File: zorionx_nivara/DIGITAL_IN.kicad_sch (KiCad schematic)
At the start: 8 parts, among them U5 LTV-357T, U6 LTV-357T

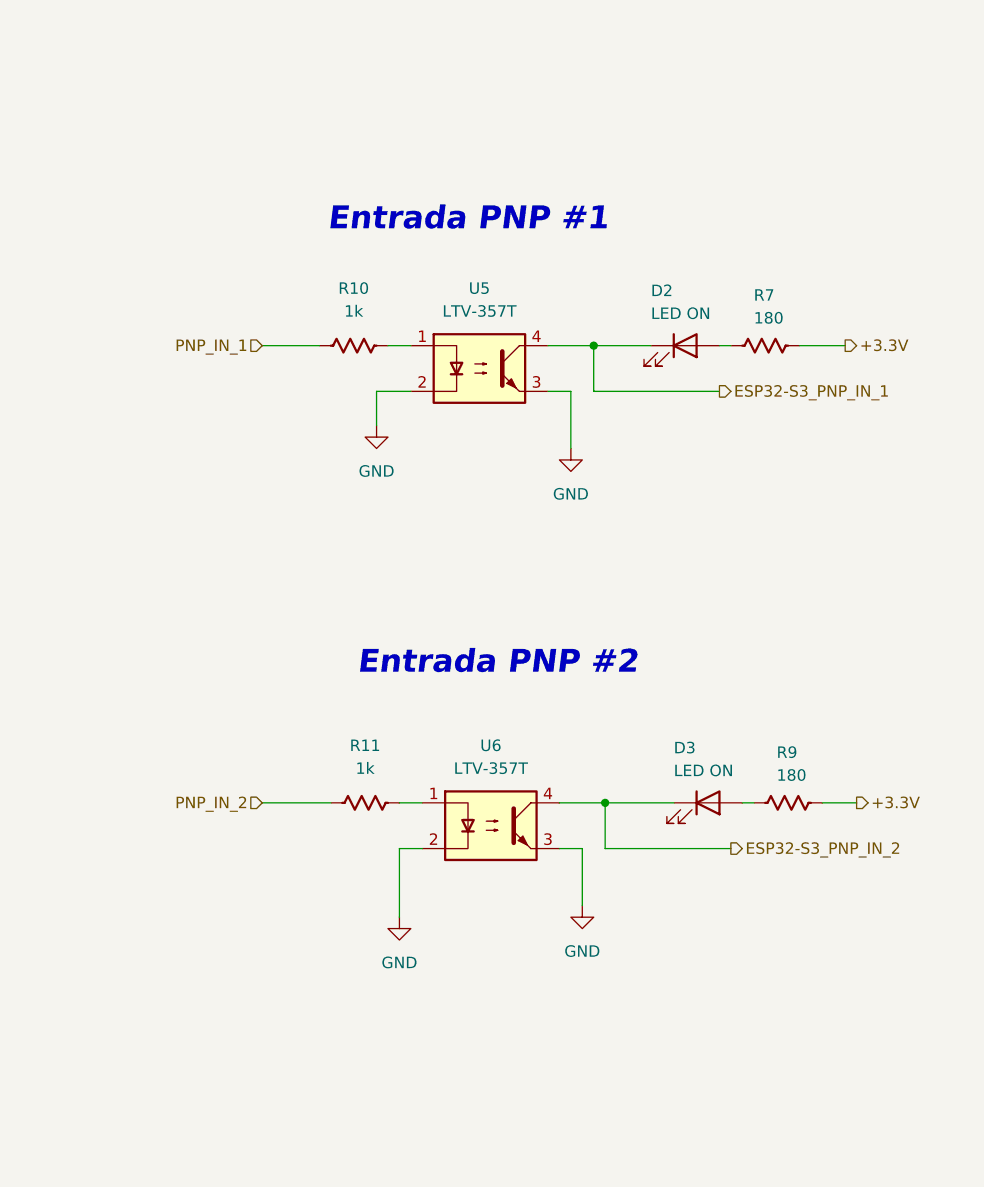
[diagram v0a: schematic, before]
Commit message: ultimo commit 1
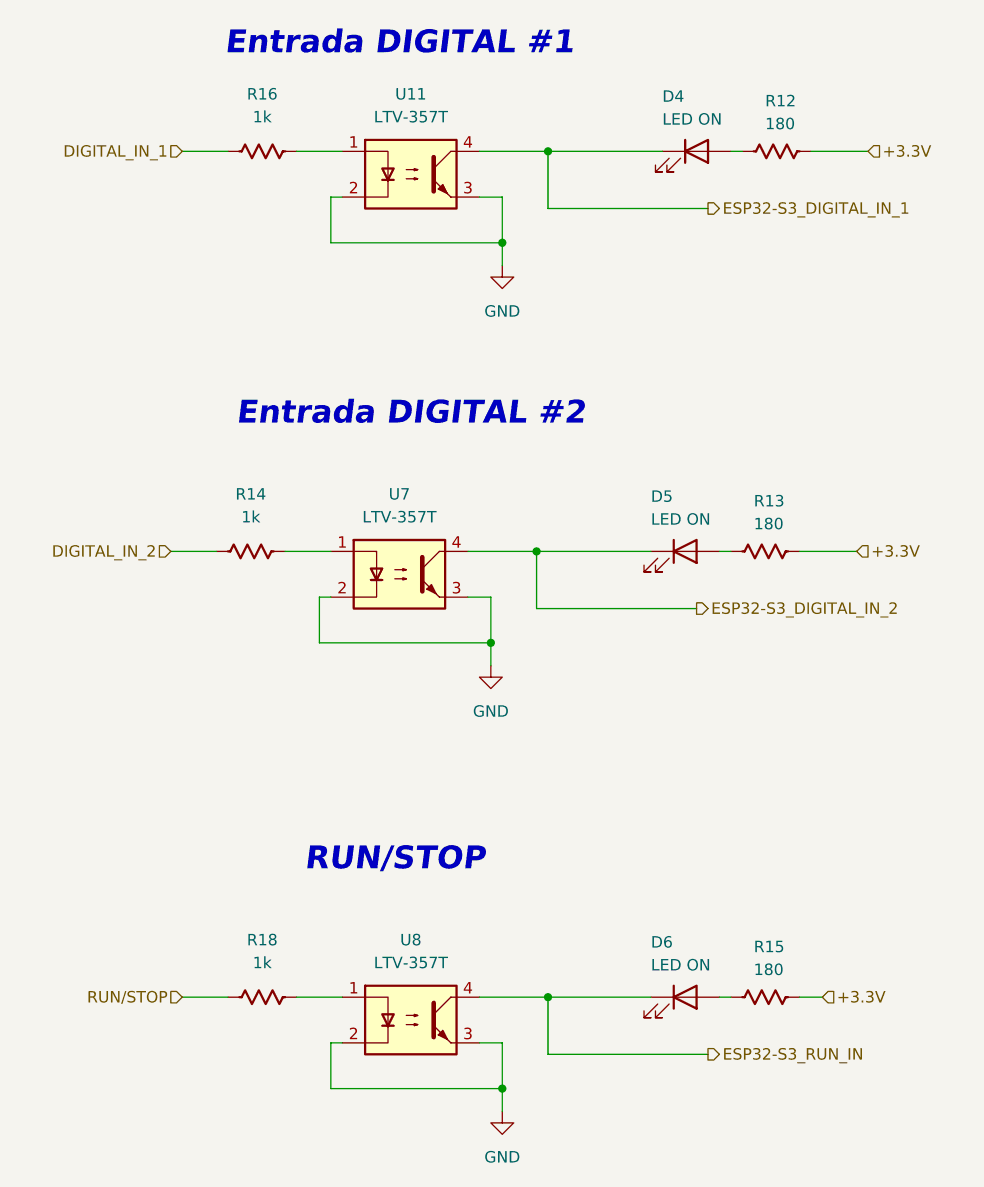
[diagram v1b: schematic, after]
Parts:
- removed D2, D3: LED ON, LED_SMD:LED_0603_1608Metric, symbol Device:LED
- removed R10, R11: 1k, PCM_Resistor_SMD_AKL:R_0603_1608Metric, symbol PCM_Resistor_US_AKL:R_0603
- removed R7, R9: 180, PCM_Resistor_SMD_AKL:R_0603_1608Metric, symbol PCM_Resistor_US_AKL:R_0603
- removed U5, U6: LTV-357T, Package_SO:SO-4_4.4x3.6mm_P2.54mm, symbol Isolator:LTV-357T
- added D4, D5, D6: LED ON, LED_SMD:LED_0603_1608Metric, symbol Device:LED
- added R12, R13, R15: 180, PCM_Resistor_SMD_AKL:R_0603_1608Metric, symbol PCM_Resistor_US_AKL:R_0603
- added R14, R16, R18: 1k, PCM_Resistor_SMD_AKL:R_0603_1608Metric, symbol PCM_Resistor_US_AKL:R_0603
- added U11, U7, U8: LTV-357T, Package_SO:SO-4_4.4x3.6mm_P2.54mm, symbol Isolator:LTV-357T
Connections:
- net +3.3V: now also R12.1, R13.1, R15.1
- net GND: now also U11.2, U11.3, U7.2, U7.3, U8.2, U8.3
- new net: R18.2, U8.1
- new net: D5.2 (A), R13.2
- new net: D4.2 (A), R12.2
- new net: R16.2, U11.1
- new net: D6.2 (A), R15.2
- new net: R14.2, U7.1
- new net DIGITAL_IN_1: R16.1
- new net DIGITAL_IN_2: R14.1
- new net ESP32-S3_DIGITAL_IN_1: D4.1 (K), U11.4
- new net ESP32-S3_DIGITAL_IN_2: D5.1 (K), U7.4
- new net ESP32-S3_RUN_IN: D6.1 (K), U8.4
- new net RUN/STOP: R18.1
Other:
- note added: "Entrada DIGITAL #1"
- note added: "Entrada DIGITAL #2"
- note added: "RUN/STOP"
- note removed: "Entrada PNP #1"
- note removed: "Entrada PNP #2"
